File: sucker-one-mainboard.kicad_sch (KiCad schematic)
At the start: 120 parts, among them J1 JST NC Valve, J10 JST Motor, J11 Conn_02x04_Odd_Even, J12 TYPE-C-31-M-12, J2 JST NO Valve, J3 6P4C, J4 JST 3 Way Valve, J5 Jack-DC, J6 Phoenix Contact 1733570, J7 QWIIC I2C, J8 SPI, J9 52271-1079, Q1 BSS138, Q2 BSS138, Q3 BSS138, Q6 STN4NF20L, U1 LD1117S33TR, Y1 ABLS-12.000MHZ-B4-T

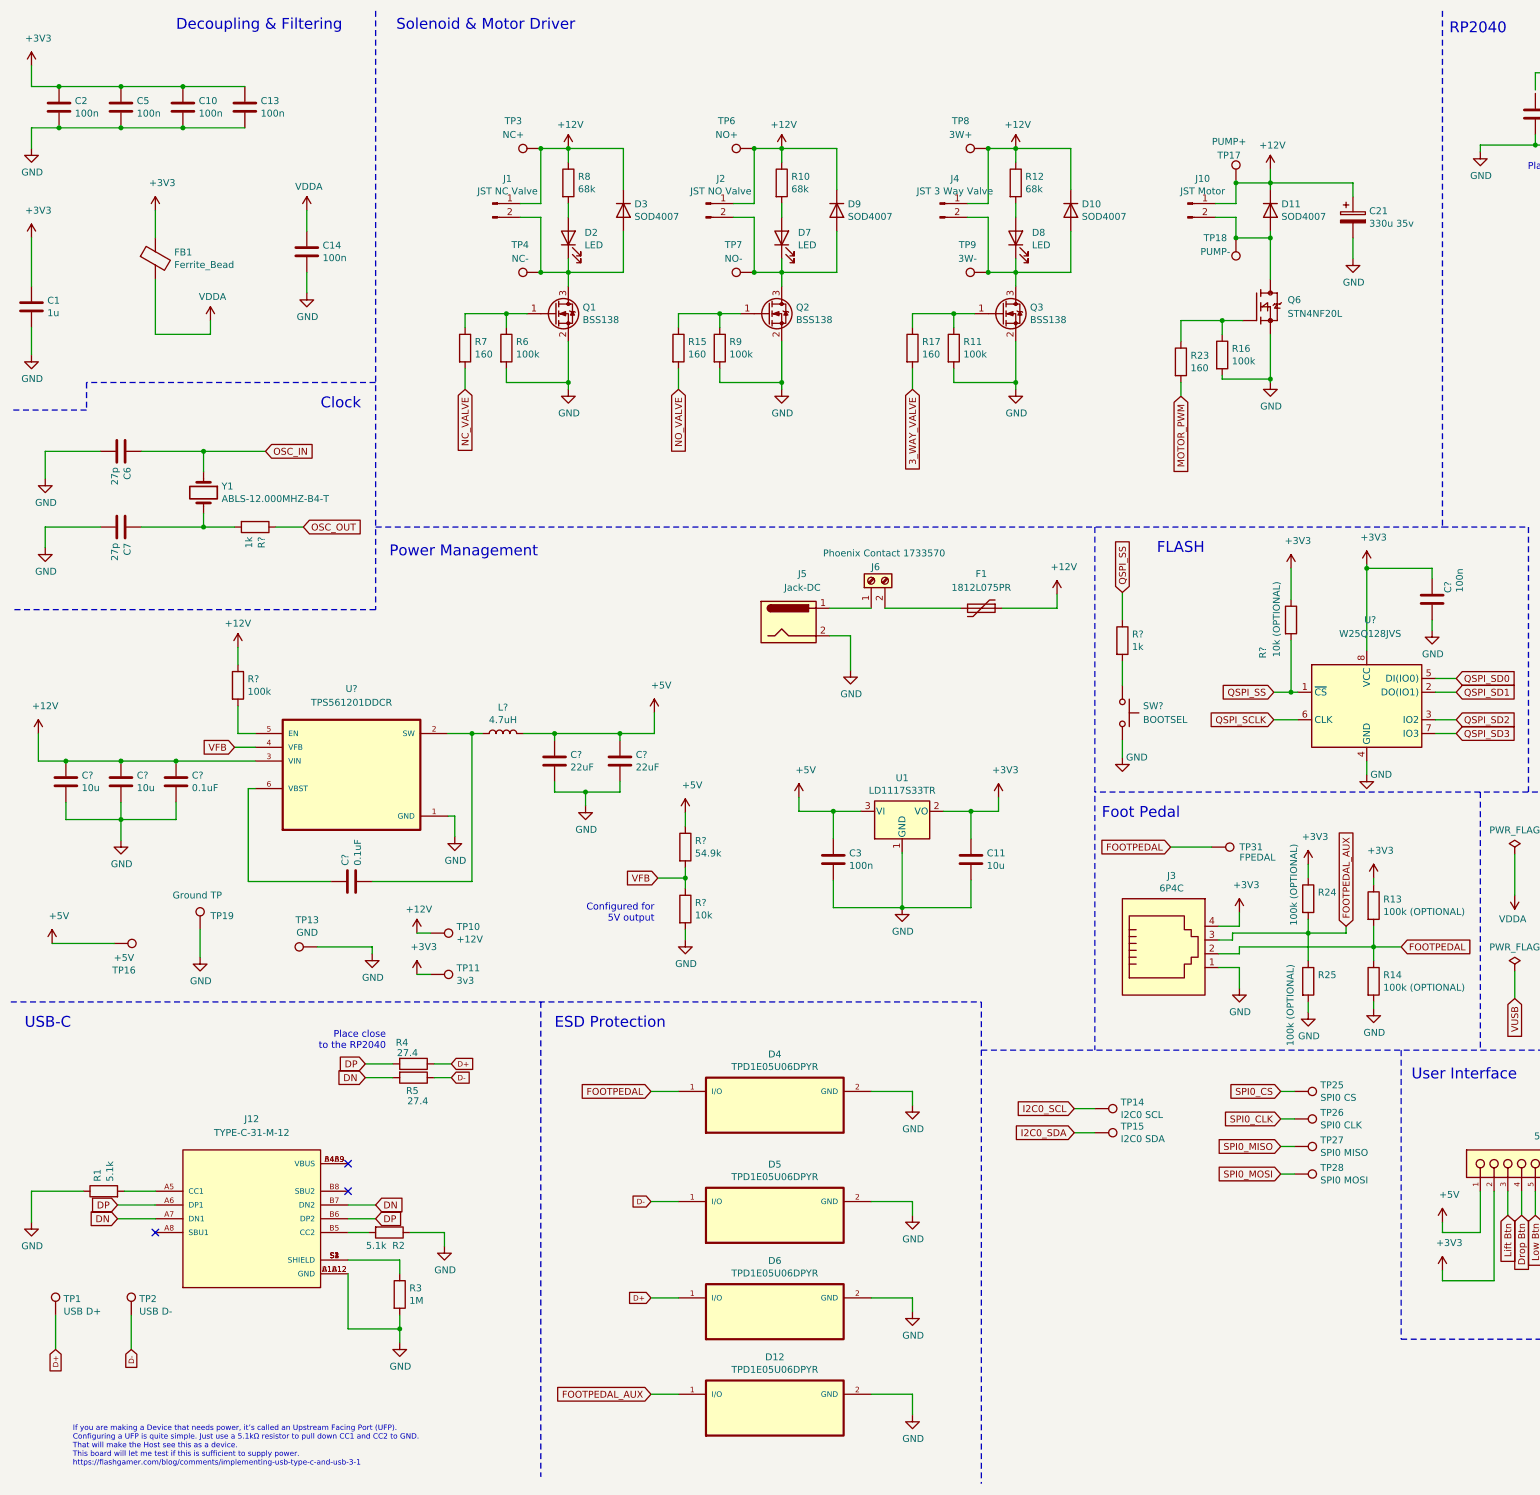
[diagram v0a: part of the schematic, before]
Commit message: Cleanup
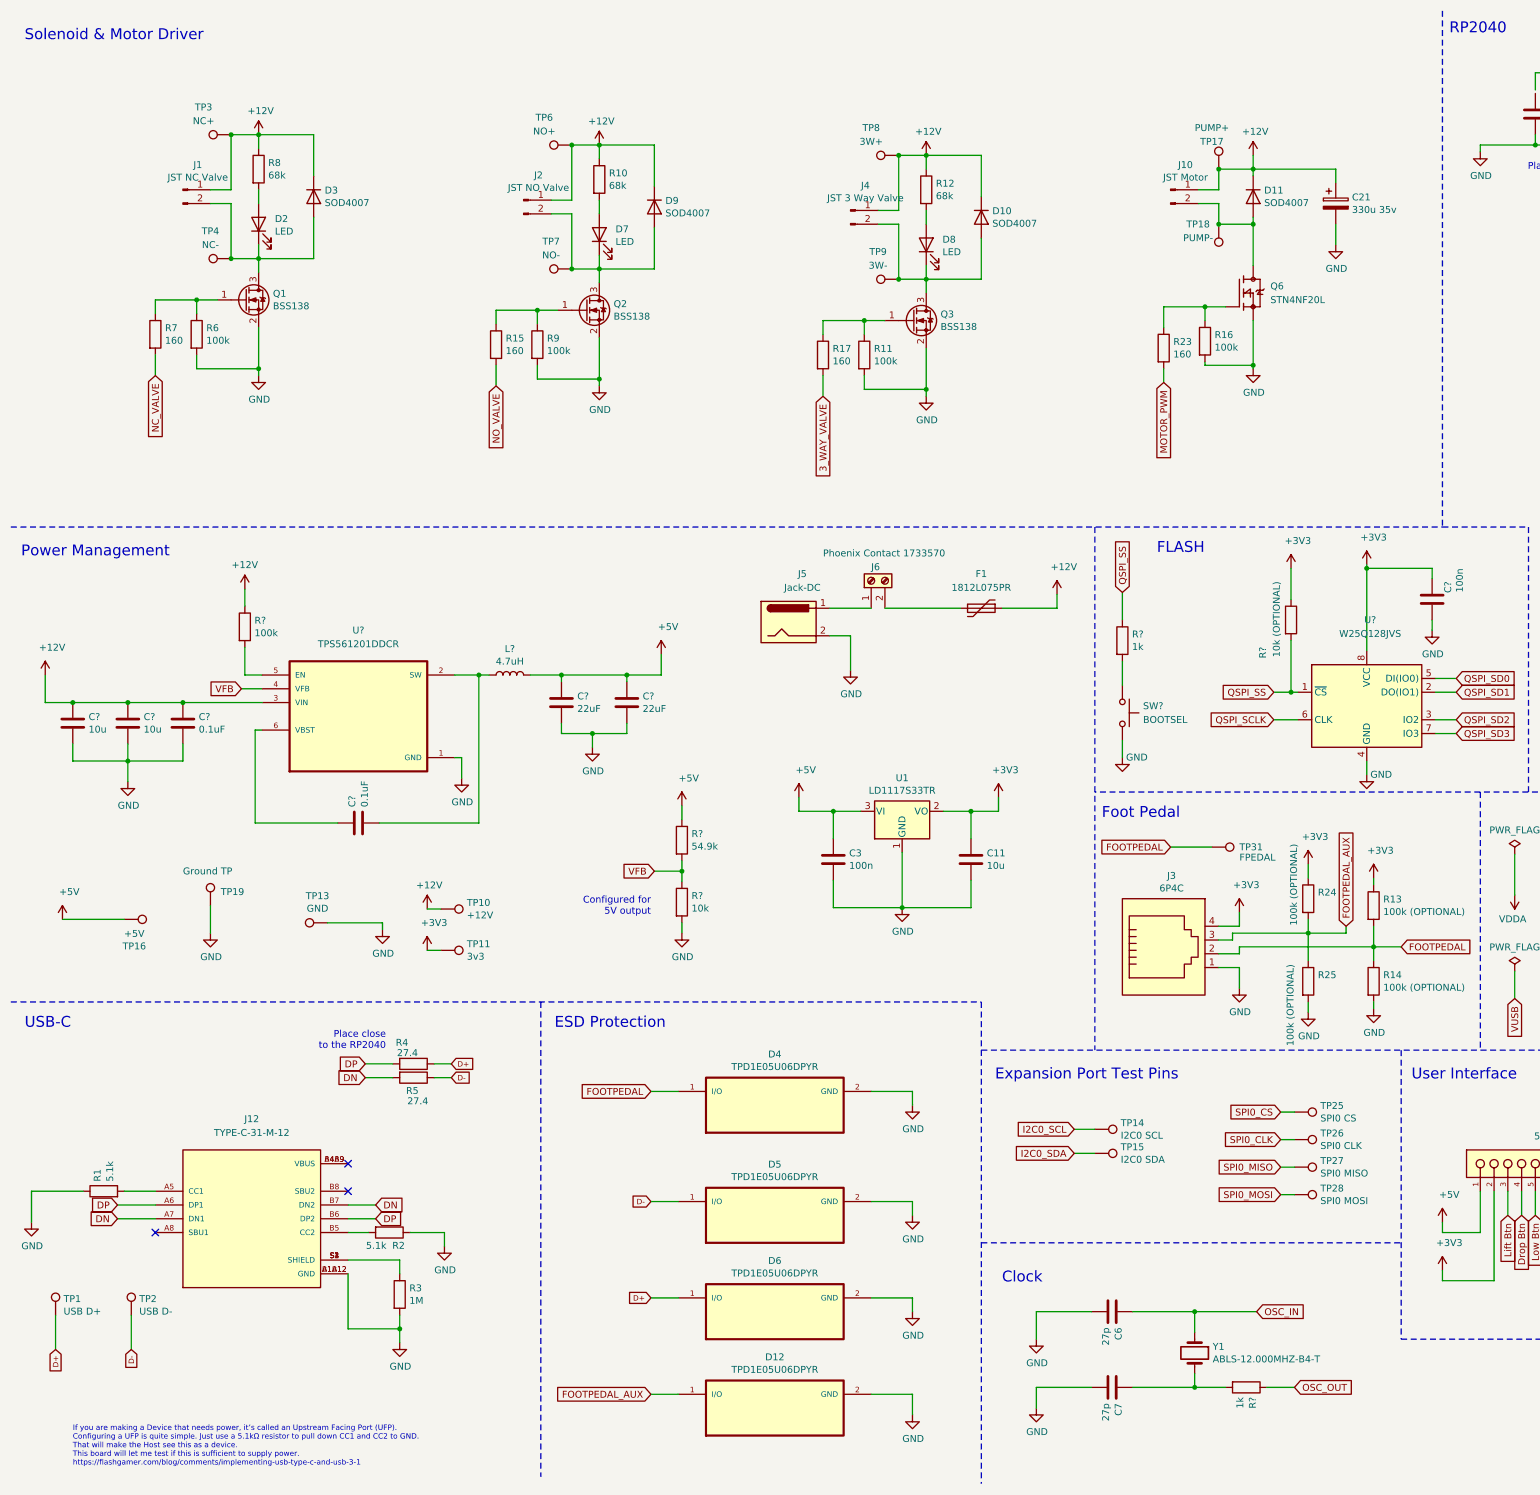
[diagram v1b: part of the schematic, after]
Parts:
- removed C1: 1u, Capacitor_SMD:C_0603_1608Metric_Pad1.08x0.95mm_HandSolder, symbol Device:C
- removed C10, C13, C14, C2, C5: 100n, Capacitor_SMD:C_0603_1608Metric_Pad1.08x0.95mm_HandSolder, symbol Device:C
- removed FB1: Ferrite_Bead, Inductor_SMD:L_0603_1608Metric_Pad1.05x0.95mm_HandSolder, symbol sucker-one-mainboard-rescue:Ferrite_Bead-Device
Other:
- note added: "Expansion Port Test Pins"
- note removed: "Decoupling & Filtering"
- moved on the sheet: C21, C6, C7, C?, D10, D11, D2, D3, D7, D8, D9, J1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
